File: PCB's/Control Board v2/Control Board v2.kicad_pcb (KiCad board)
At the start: 2 copper layers, 93 x 67.5 mm, 39 parts, among them J1 Power In, J2 LED Strip Conn, J3 Expansion, J4 Expansion, SW1 SW_Push, SW2 SW_Push, SW3 SW_Push, SW4 SW_Push, SW5 SW_Push, SW6 SW_Push, SW7 SW_Push, SW8 SW_Push, U1 ESP32-DEVKITC-32E, U2 L7805, U3 TXS0101DBV, U4 TXS0101DBV, U5 TXS0101DBV, U6 CD74HC4051M96

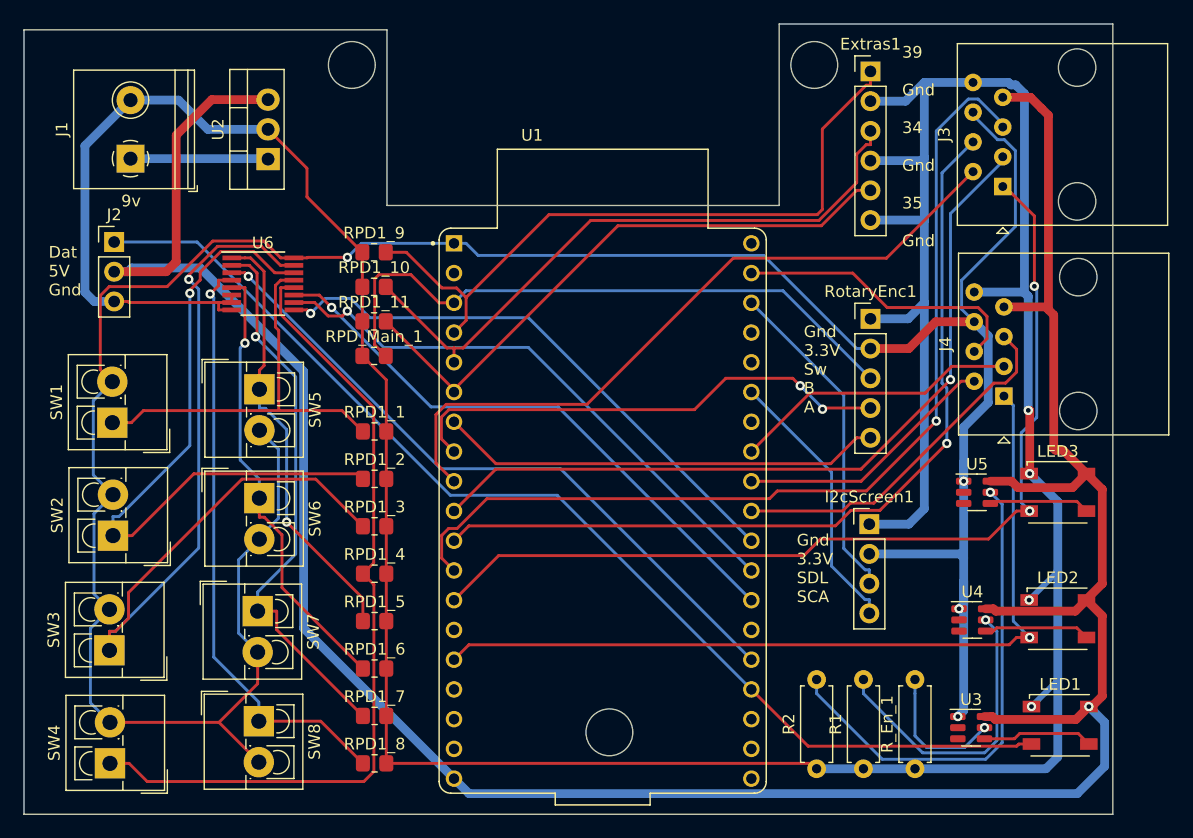
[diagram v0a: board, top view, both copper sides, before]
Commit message: updates
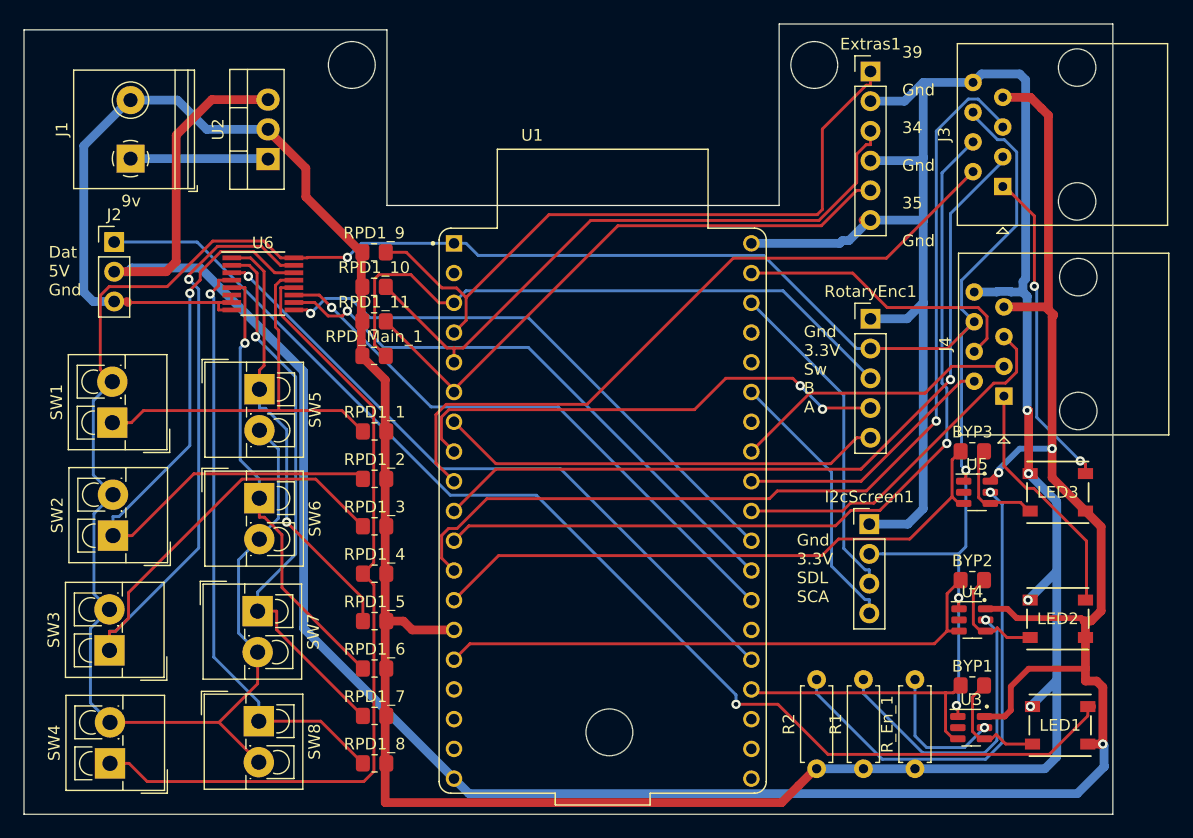
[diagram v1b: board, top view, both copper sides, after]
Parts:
- added BYP1: ~, Resistor_SMD:R_0805_2012Metric_Pad1.20x1.40mm_HandSolder, F.Cu at (110.0, 85.0)
- added BYP2: ~, Resistor_SMD:R_0805_2012Metric_Pad1.20x1.40mm_HandSolder, F.Cu at (110.0, 76.0)
- added BYP3: ~, Resistor_SMD:R_0805_2012Metric_Pad1.20x1.40mm_HandSolder, F.Cu at (110.0, 65.0)
- LED1, LED2, LED3: footprint LED_SMD:LED_Inolux_IN-PI554FCH_PLCC4_5.0x5.0mm_P3.2mm -> Relay_parts:LED_IN-PI55TAT_INL
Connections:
- U1 pad J2_13: LED_3_Data -> LED_3_sig
- U1 pad J2_14: unconnected-(U1-GND_J2_14-PadJ2_14) -> GND
- U1 pad J2_15: LED_2_Data -> LED_2_sig
- U1 pad J3_1: unconnected-(U1-GND_J3_1-PadJ3_1) -> GND
- U1 pad J3_16: LED_1_Data -> LED_1_sig
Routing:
- net LED_3_Data: track 82.2 -> 28.0 mm
- net LED_3_sig: track 0.00 -> 51.6 mm
- net LED_2_Data: track 71.5 -> 20.8 mm, vias 1 -> 0
- net LED_2_sig: track 0.00 -> 49.0 mm
- net GND: track 302.1 -> 330.2 mm
- net LED_1_sig: track 0.00 -> 22.8 mm
- net LED_1_Data: track 96.3 -> 104.3 mm, vias 0 -> 1
- net +3.3V: track 236.1 -> 232.8 mm
- net Net-(LED1-DIN): track 9.47 -> 10.5 mm
- net Net-(LED2-DIN): track 9.07 -> 9.68 mm
- net +5V: track 238.8 -> 239.3 mm, vias 1 -> 3
